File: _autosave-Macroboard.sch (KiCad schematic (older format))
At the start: 34 parts, among them SW1 SW_Push, U1 ATmega32U4-AU, Y1 16MHz

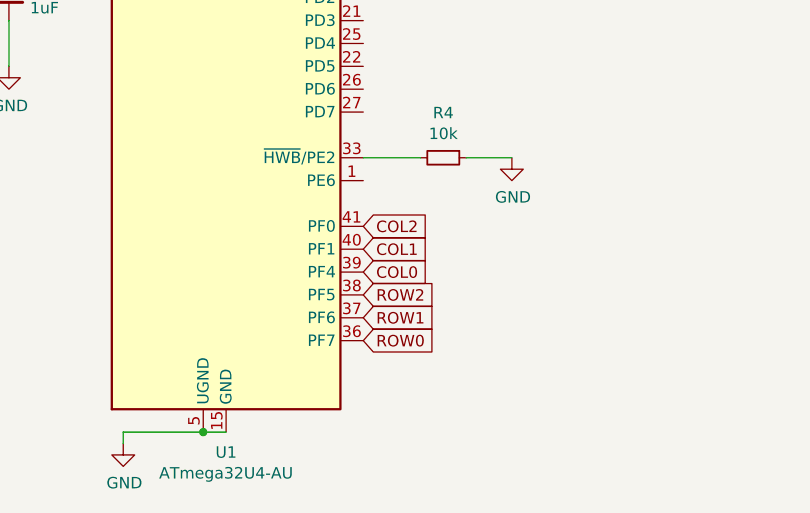
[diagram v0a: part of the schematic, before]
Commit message: PCB v1 done
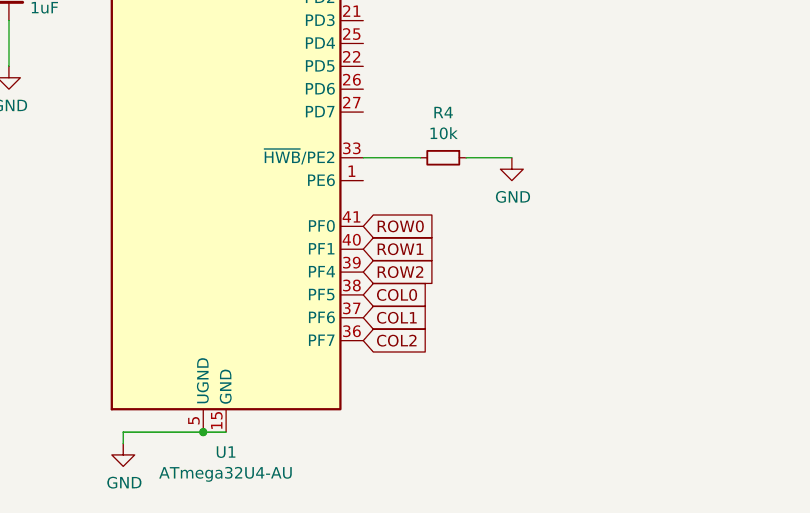
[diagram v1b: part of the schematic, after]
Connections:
- net COL0: now also U1.38 (PF5); no longer U1.39 (PF4)
- net COL1: now also U1.37 (PF6); no longer U1.40 (PF1)
- net COL2: now also U1.36 (PF7); no longer U1.41 (PF0)
- net ROW0: now also U1.41 (PF0); no longer U1.36 (PF7)
- net ROW1: now also U1.40 (PF1); no longer U1.37 (PF6)
- net ROW2: now also U1.39 (PF4); no longer U1.38 (PF5)
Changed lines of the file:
@@
 Text GLabel 7750 3650 0    50   Input ~ 0
 ROW2
+Text GLabel 4200 5800 2    50   Input ~ 0
+ROW0
+Text GLabel 4200 5900 2    50   Input ~ 0
+ROW1
+Text GLabel 4200 6000 2    50   Input ~ 0
+ROW2
+Text GLabel 4200 6100 2    50   Input ~ 0
+COL0
+Text GLabel 4200 6200 2    50   Input ~ 0
+COL1
 Text GLabel 4200 6300 2    50   Input ~ 0
-ROW0
-Text GLabel 4200 6200 2    50   Input ~ 0
-ROW1
-Text GLabel 4200 6100 2    50   Input ~ 0
-ROW2
-Text GLabel 4200 6000 2    50   Input ~ 0
-COL0
-Text GLabel 4200 5900 2    50   Input ~ 0
-COL1
-Text GLabel 4200 5800 2    50   Input ~ 0
 COL2
 $EndSCHEMATC
